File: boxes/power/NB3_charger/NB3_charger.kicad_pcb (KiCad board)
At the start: 2 copper layers, 110 x 71 mm, 40 parts, among them J1 Barrel_Jack_PJ-036AH-SMT-TR, J2 Connector_S4B-PH-SM4-TB(LF)(S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, J3 Conn_01x02_Pin, SW1 SW_SPDT, U1 Voltage_Regulator_AP64501

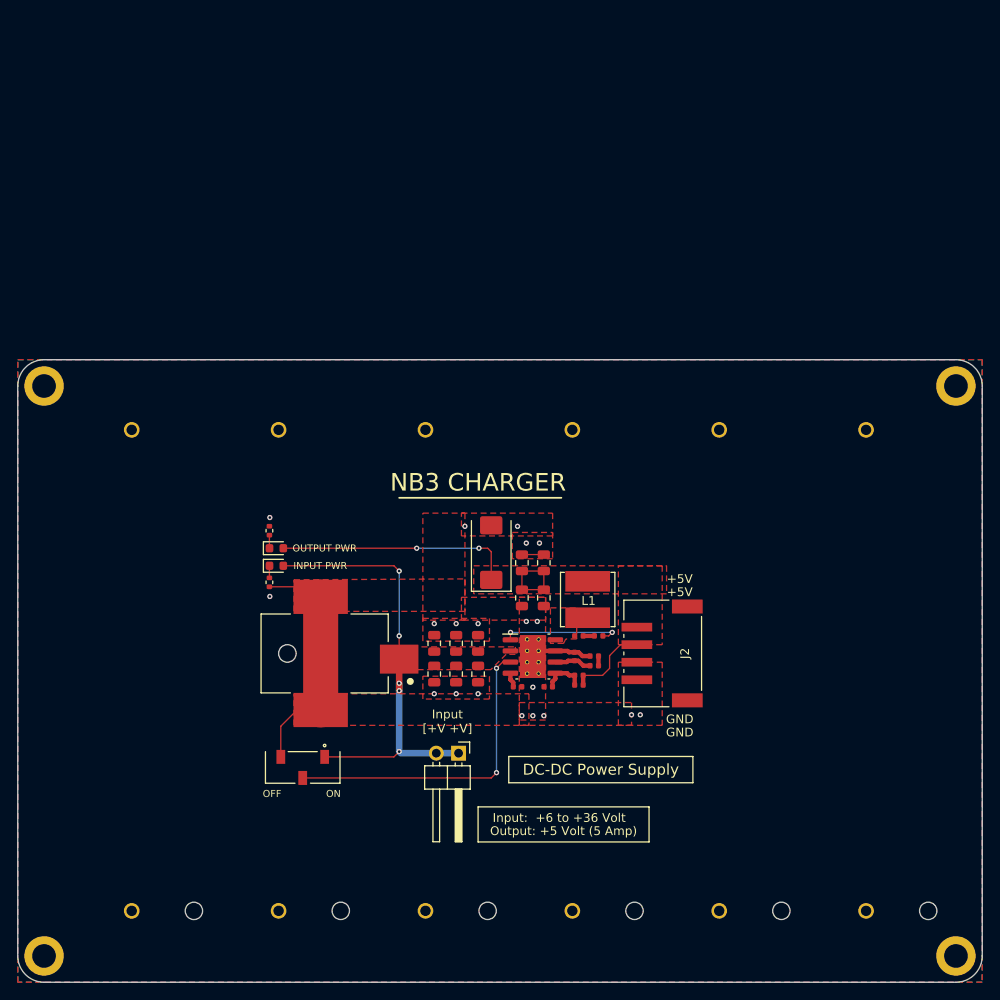
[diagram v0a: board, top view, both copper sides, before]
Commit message: Work on PCBs (v1 and v2)
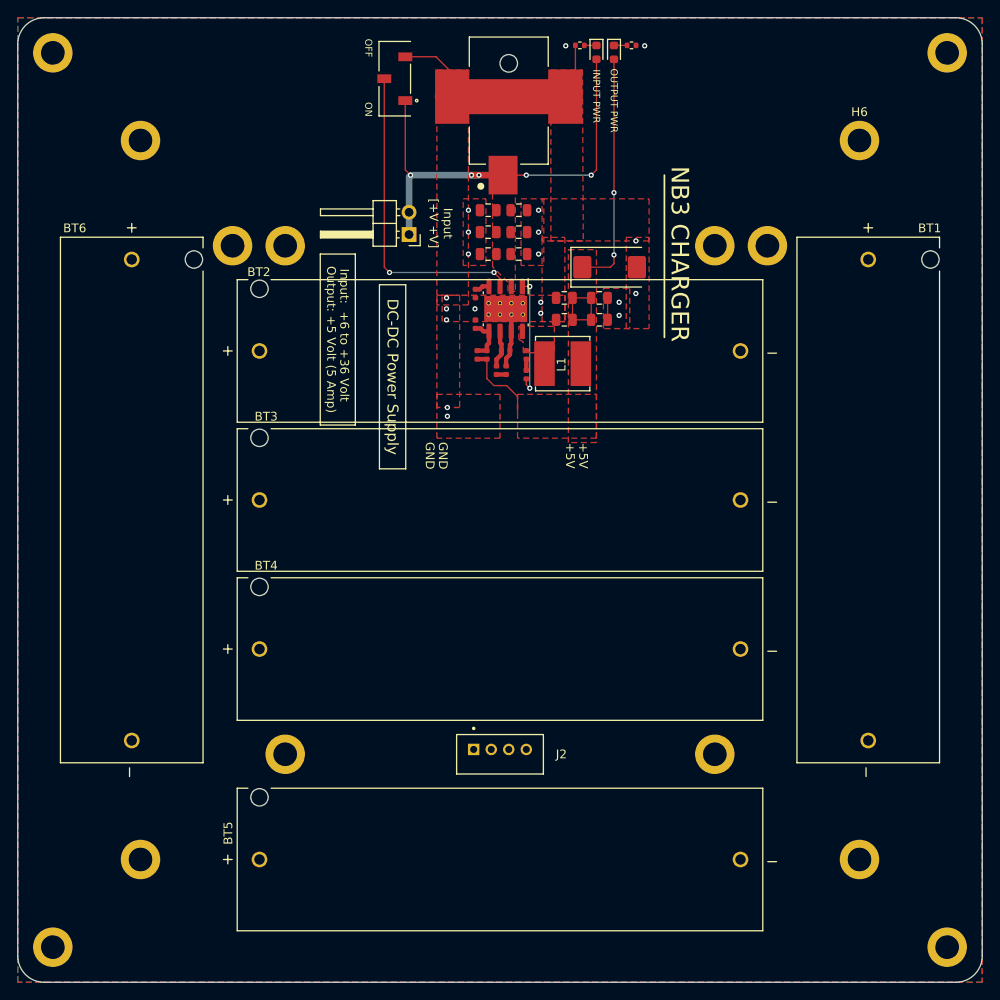
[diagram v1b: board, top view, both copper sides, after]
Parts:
- added H10: MountingHole, MountingHole:MountingHole_2.7mm_M2.5_ISO7380_Pad, F.Cu at (209.5, 46.2)
- added H11: MountingHole, MountingHole:MountingHole_2.7mm_M2.5_ISO7380_Pad, F.Cu at (209.5, 104.2)
- added H12: MountingHole, MountingHole:MountingHole_2.7mm_M2.5_ISO7380_Pad, F.Cu at (160.5, 104.2)
- added H13: MountingHole, MountingHole:MountingHole_2.7mm_M2.5_ISO7380_Pad, F.Cu at (154.5, 46.2)
- added H14: MountingHole, MountingHole:MountingHole_2.7mm_M2.5_ISO7380_Pad, F.Cu at (215.5, 46.2)
- added H5: MountingHole, MountingHole:MountingHole_2.7mm_M2.5_ISO7380_Pad, F.Cu at (144.0, 34.2)
- added H6: MountingHole, MountingHole:MountingHole_2.7mm_M2.5_ISO7380_Pad, F.Cu at (226.0, 34.2)
- added H7: MountingHole, MountingHole:MountingHole_2.7mm_M2.5_ISO7380_Pad, F.Cu at (226.0, 116.2)
- added H8: MountingHole, MountingHole:MountingHole_2.7mm_M2.5_ISO7380_Pad, F.Cu at (144.0, 116.2)
- added H9: MountingHole, MountingHole:MountingHole_2.7mm_M2.5_ISO7380_Pad, F.Cu at (160.5, 46.2)
- BT1, BT2, BT3, BT4, BT5, BT6: moved to F.Cu
- J2: value Connector_S4B-PH-SM4-TB(LF)(SN) -> B4B-PH-K-S; footprint NB3_charger:Connector_S4B-PH-SM4-TB(LF)(SN) -> NB3_charger:Connector_B4B-PH-K-S(LF)(SN)
- moved H3 121.3 mm to (236.0, 126.2), turned to 0 degrees
- moved H1 109.8 mm to (134.0, 24.2), turned to 0 degrees
- moved H2 103.0 mm to (236.0, 24.2), turned to 0 degrees
- moved BT1 86.2 mm to (227.0, 75.2), turned to -90 degrees
- moved BT6 86.0 mm to (143.0, 75.2), turned to -90 degrees
- moved SW1 79.2 mm to (173.0, 27.2), turned to 90 degrees
- moved R1 70.7 mm to (194.1, 23.4), turned to 180 degrees
- moved R6 69.1 mm to (200.0, 23.4), turned to 0 degrees
- moved D1 69.0 mm to (196.0, 24.2), turned to -90 degrees
- moved D2 68.4 mm to (198.0, 24.2), turned to -90 degrees
- moved J3 59.4 mm to (174.6, 45.0), turned to 180 degrees
- moved J1 56.5 mm to (185.3, 38.2), turned to -90 degrees
- moved C3 53.3 mm to (183.7, 42.2), turned to 180 degrees
- moved C1 50.5 mm to (183.7, 44.7), turned to 180 degrees
- moved C4 50.3 mm to (187.2, 42.2), turned to 0 degrees
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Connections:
- J2 pad 1: GND -> +5V
- J2 pad 2: GND -> +5V
- J2 pad 3: +5V -> GND
- J2 pad 4: +5V -> GND
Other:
- board size 110 x 71 mm -> 110 x 110 mm
